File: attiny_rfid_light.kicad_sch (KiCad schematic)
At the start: 27 parts, among them IC1 EM4095, U1 ESP32-WROOM-32, U2 NCP1117-3.3_SOT223

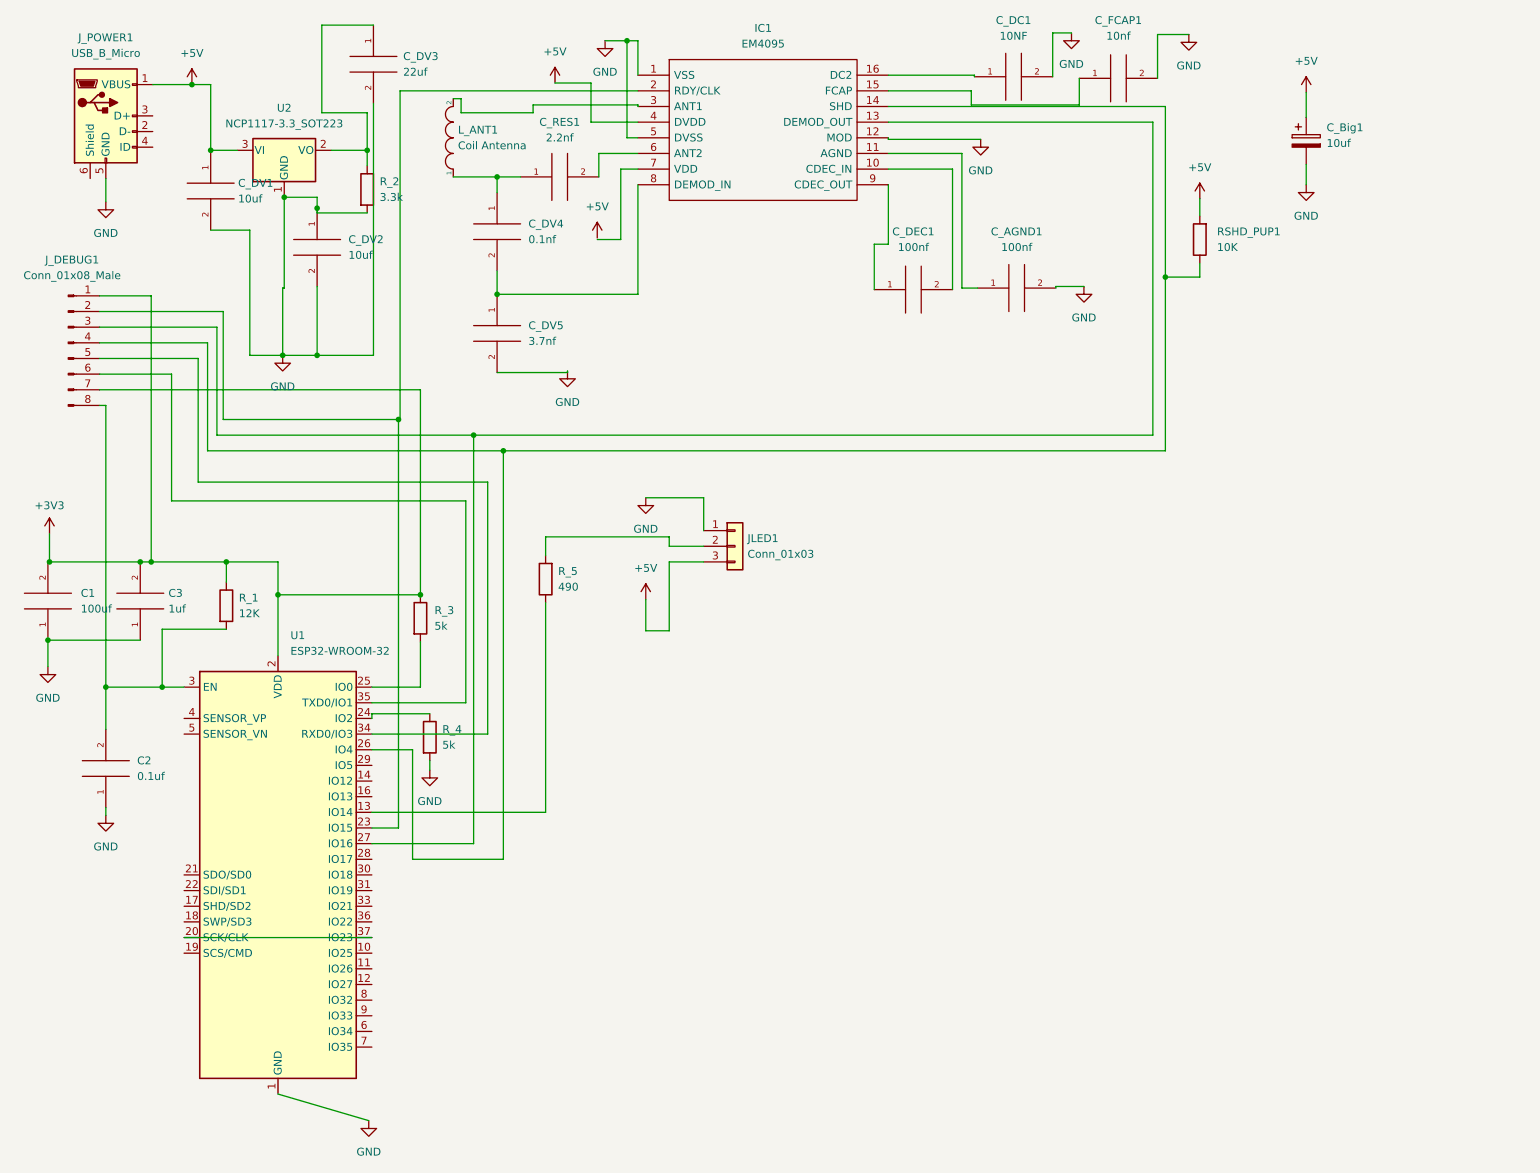
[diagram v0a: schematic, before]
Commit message: v3
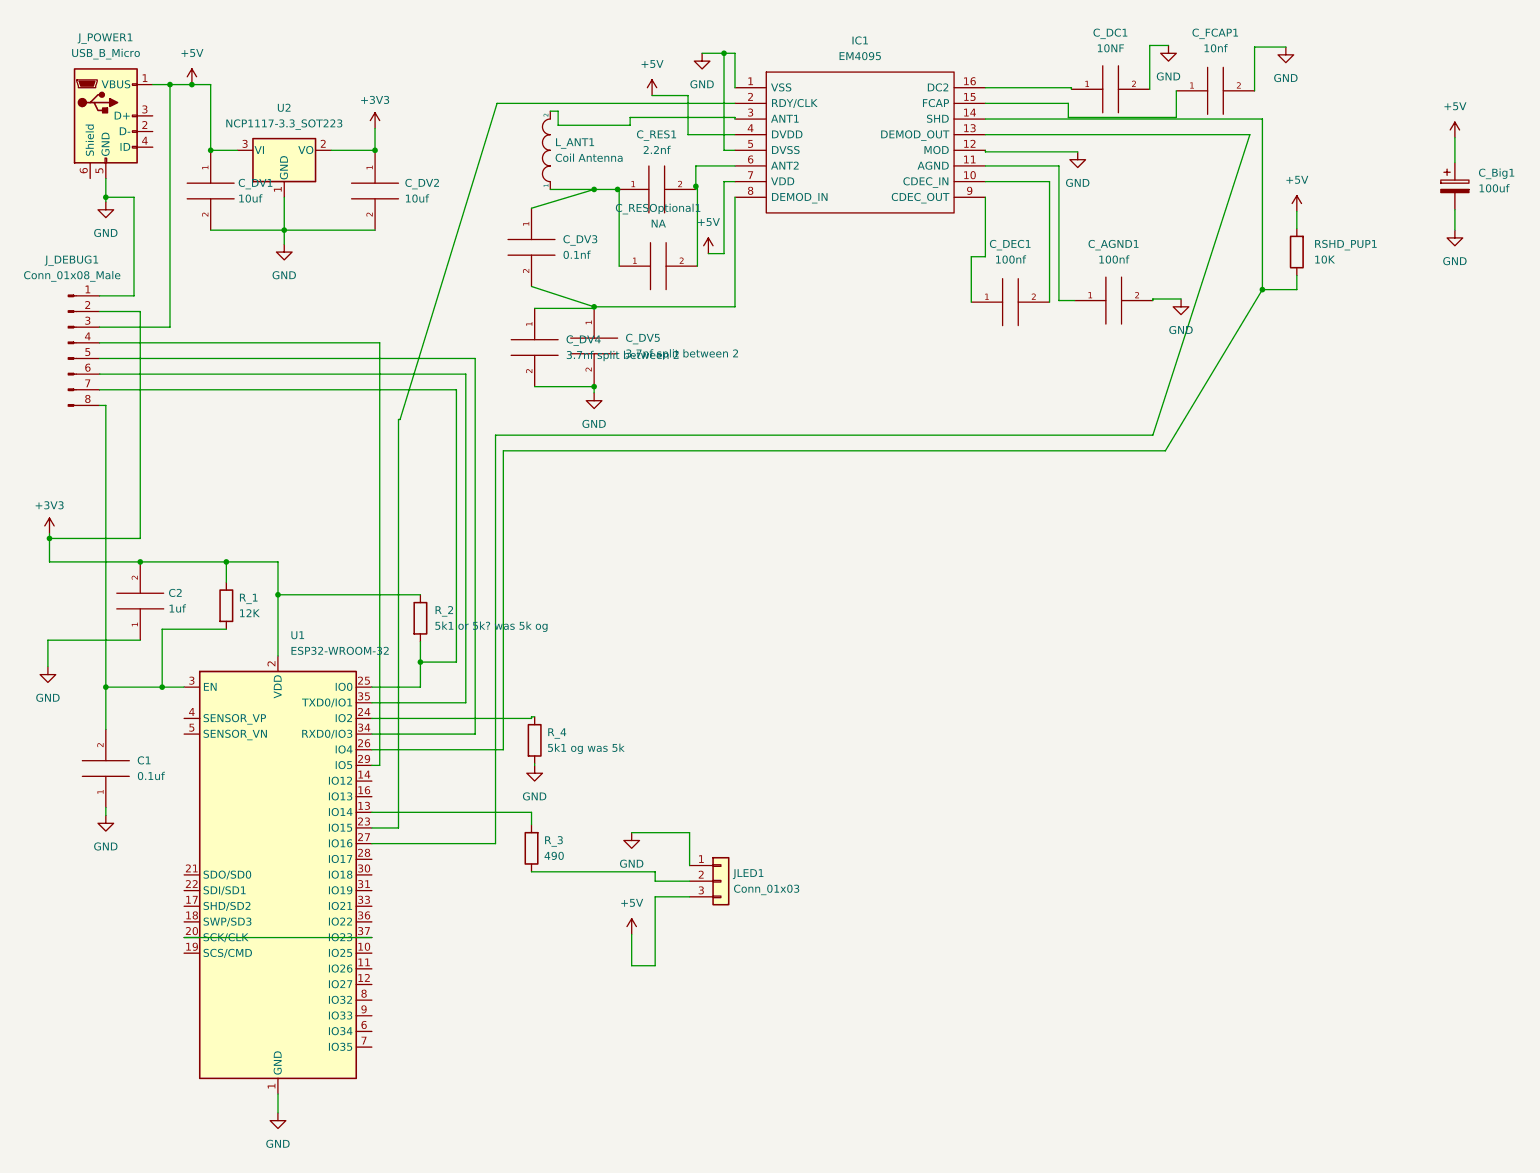
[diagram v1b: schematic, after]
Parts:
- removed C1: 100uf, Capacitor_SMD:C_0805_2012Metric_Pad1.18x1.45mm_HandSolder, symbol pspice:C
- removed C_DV2: 10uf, Capacitor_SMD:C_0805_2012Metric_Pad1.18x1.45mm_HandSolder, symbol pspice:C
- removed R_2: 3.3k, Resistor_SMD:R_0805_2012Metric_Pad1.20x1.40mm_HandSolder, symbol Device:R
- added C_DV4: 3.7nf split between 2, Capacitor_SMD:C_0805_2012Metric_Pad1.18x1.45mm_HandSolder, symbol pspice:C
- added C_RESOptional1: NA, Capacitor_SMD:C_0805_2012Metric_Pad1.18x1.45mm_HandSolder, symbol pspice:C
- C_Big1: value 10uf -> 100uf
- C_DV2: renamed from C_DV3; value 22uf -> 10uf
- C_DV5: value 3.7nf -> 3.7nf split between 2
- R_2: renamed from R_3; value 5k -> 5k1 or 5k? was 5k og
- R_4: value 5k -> 5k1 og was 5k
- renumbered C2 to C1, C3 to C2, C_DV4 to C_DV3, R_5 to R_3
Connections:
- net +3V3: now also C_DV2.1, J_DEBUG1.2 (Pin_2), U2.2 (VO); no longer J_DEBUG1.1 (Pin_1), J_DEBUG1.7 (Pin_7)
- net +5V: now also IC1.7 (VDD), J_DEBUG1.3 (Pin_3)
- net GND: now also J_DEBUG1.1 (Pin_1), C_DV4.2
- net at IC1.2 (RDY/CLK), U1.23 (IO15): no longer J_DEBUG1.2 (Pin_2)
- net at IC1.13 (DEMOD_OUT), U1.27 (IO16): no longer J_DEBUG1.3 (Pin_3)
- net at IC1.14 (SHD), RSHD_PUP1.1, U1.26 (IO4): no longer J_DEBUG1.4 (Pin_4)
- net at C_DV3.2, C_DV5.1, IC1.8 (DEMOD_IN): now also C_DV4.1
- net at C_RES1.2, IC1.6 (ANT2): now also C_RESOptional1.2
- net at C_DV3.1, C_RES1.1, L_ANT1.1: now also C_RESOptional1.1
- net at JLED1.2 (Pin_2): now also R_3.1; no longer R_3.2
- net at U1.13 (IO14): now also R_3.2; no longer R_3.1
- net at R_2.2, U1.25 (IO0): now also J_DEBUG1.7 (Pin_7)
- net at U1.29 (IO5): now also J_DEBUG1.4 (Pin_4)
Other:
- moved on the sheet: C_AGND1, C_Big1, C_DC1, C_DEC1, C_DV2, C_DV3, C_DV5, C_FCAP1, C_RES1, IC1, JLED1, L_ANT1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
